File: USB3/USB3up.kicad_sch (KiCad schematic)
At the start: 5 parts

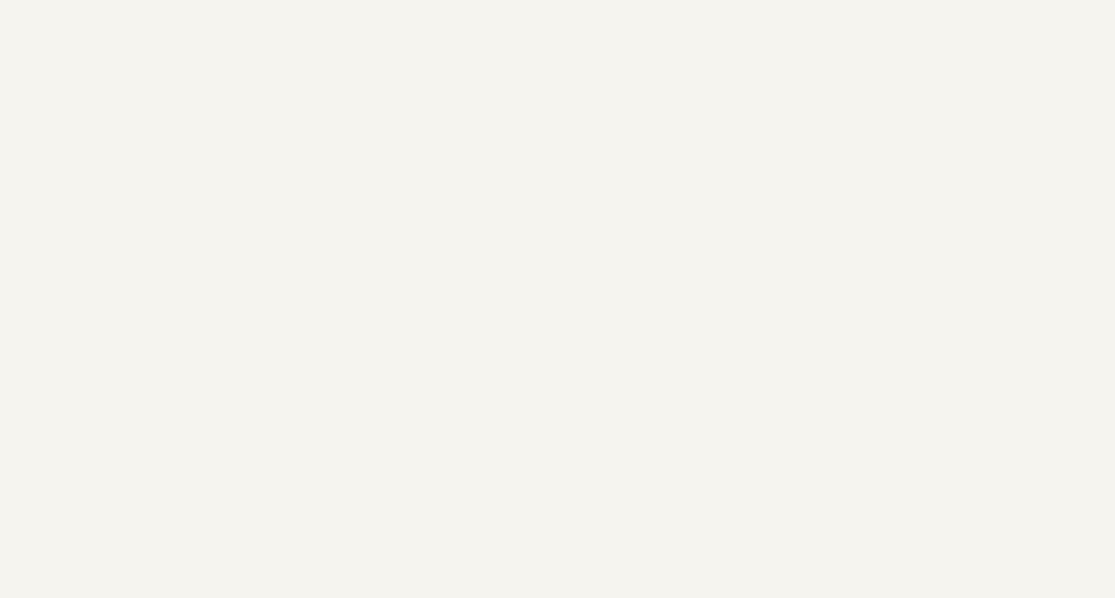
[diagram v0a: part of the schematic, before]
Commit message: merge test
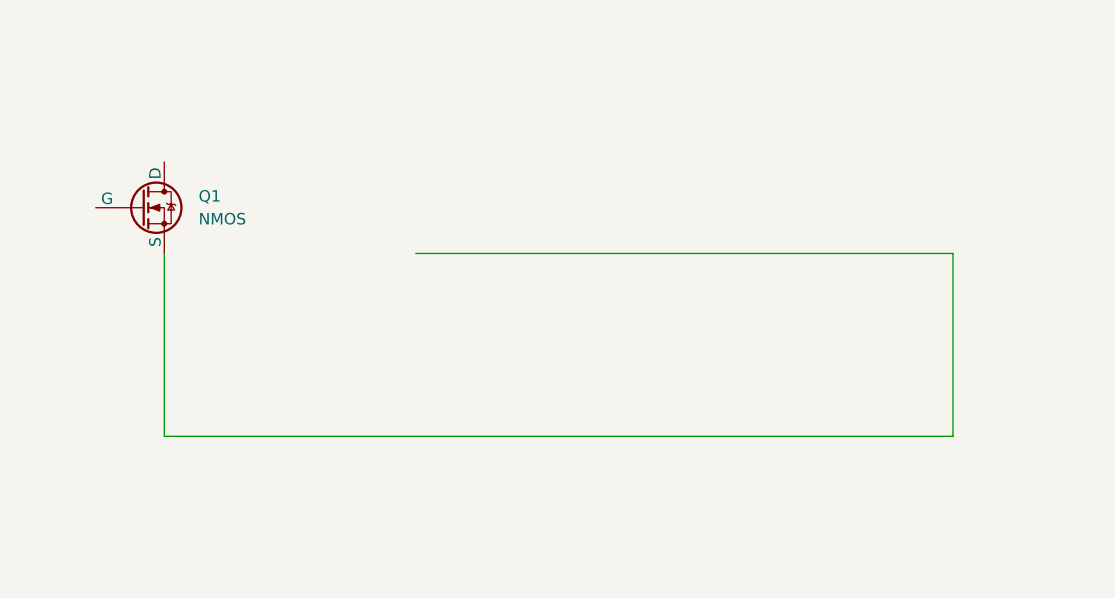
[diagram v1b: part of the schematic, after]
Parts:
- added Q1: NMOS, symbol Simulation_SPICE:NMOS
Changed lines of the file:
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@@
+	(wire
+		(pts
+			(xy 187.96 86.36) (xy 187.96 106.68)
+		)
+		(stroke
+			(width 0)
+			(type default)
+		)
+	)
 	(wire
 		(pts
@@
 		(pts
 			(xy 274.32 133.35) (xy 274.32 132.08)
+		)
+		(stroke
+			(width 0)
+			(type default)
+		)
+	)
+	(wire
+		(pts
+			(xy 128.27 86.36) (xy 187.96 86.36)
+		)
+		(stroke
+			(width 0)
+			(type default)
+		)
+	)
+	(wire
+		(pts
+			(xy 187.96 106.68) (xy 100.33 106.68)
+		)
+		(stroke
+			(width 0)
+			(type default)
+		)
+	)
+	(wire
+		(pts
+			(xy 100.33 106.68) (xy 100.33 86.36)
 		)
 		(stroke
@@
 					(unit 1)
 				)
+			)
+		)
+	)
+	(symbol
+		(lib_id "Simulation_SPICE:NMOS")
+		(at 97.79 81.28 0)
+		(unit 1)
+		(exclude_from_sim no)
+		(in_bom yes)
+		(on_board yes)
+		(dnp no)
+		(fields_autoplaced yes)
+		(property "Reference" "Q1"
+			(at 104.14 80.0099 0)
+			(effects
+				(font
+					(size 1.27 1.27)
+				)
+				(justify left)
+			)
+		)
+		(property "Value" "NMOS"
+			(at 104.14 82.5499 0)
+			(effects
+				(font
+					(size 1.27 1.27)
+				)
+				(justify left)
+			)
+		)
+		(property "Footprint" ""
+			(at 102.87 78.74 0)
+			(effects
+				(font
+					(size 1.27 1.27)
+				)
+				(hide yes)
+			)
+		)
+		(property "Datasheet" "https://ngspice.sourceforge.io/docs/ngspice-html-manual/manual.xhtml#cha_MOSFETs"
+			(at 97.79 93.98 0)
+			(effects
+				(font
+					(size 1.27 1.27)
+				)
+				(hide yes)
+			)
+		)
+		(property "Description" "N-MOSFET transistor, drain/source/gate"
+			(at 97.79 81.28 0)
+			(effects
+				(font
+					(size 1.27 1.27)
+				)
+				(hide yes)
+			)
+		)
+		(property "Sim.Device" "NMOS"
+			(at 97.79 98.425 0)
+			(effects
+				(font
+					(size 1.27 1.27)
+				)
+				(hide yes)
+			)
+		)
+		(property "Sim.Type" "VDMOS"
+			(at 97.79 100.33 0)
+			(effects
+				(font
+					(size 1.27 1.27)
+				)
+				(hide yes)
+			)
+		)
+		(property "Sim.Pins" "1=D 2=G 3=S"
+			(at 97.79 96.52 0)
+			(effects
+				(font
+					(size 1.27 1.27)
+				)
+				(hide yes)
+			)
+		)
+		(pin "1"
+		)
+		(pin "2"
+		)
+		(pin "3"
+		)
+		(instances
+			(project ""
+				(path "/600da949-f681-489f-915b-075a1ebe377b/f20b1b5c-052b-4ece-8190-313324529590/b8f6ff93-8254-477a-8cbd-4a45901a01e5"
+					(reference "Q1")
+					(unit 1)
+				)
